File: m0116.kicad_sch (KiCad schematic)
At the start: 259 parts, among them J2 Conn_01x04_MountingPin, J3 Conn_01x04_MountingPin, Q1 Q_PMOS_GSD AO3401A, Q2 Q_NMOS_GSD 2N7002, Q3 Q_NMOS_GSD 2N7002, Q4 2N3904, SW1 SW_Push, U1 XC6206P332MR, U2 74AHCT1G125, U3 STM32F411RETx, U4 24LC64, U5 USBLC6-2SC6, Y1 8MHz

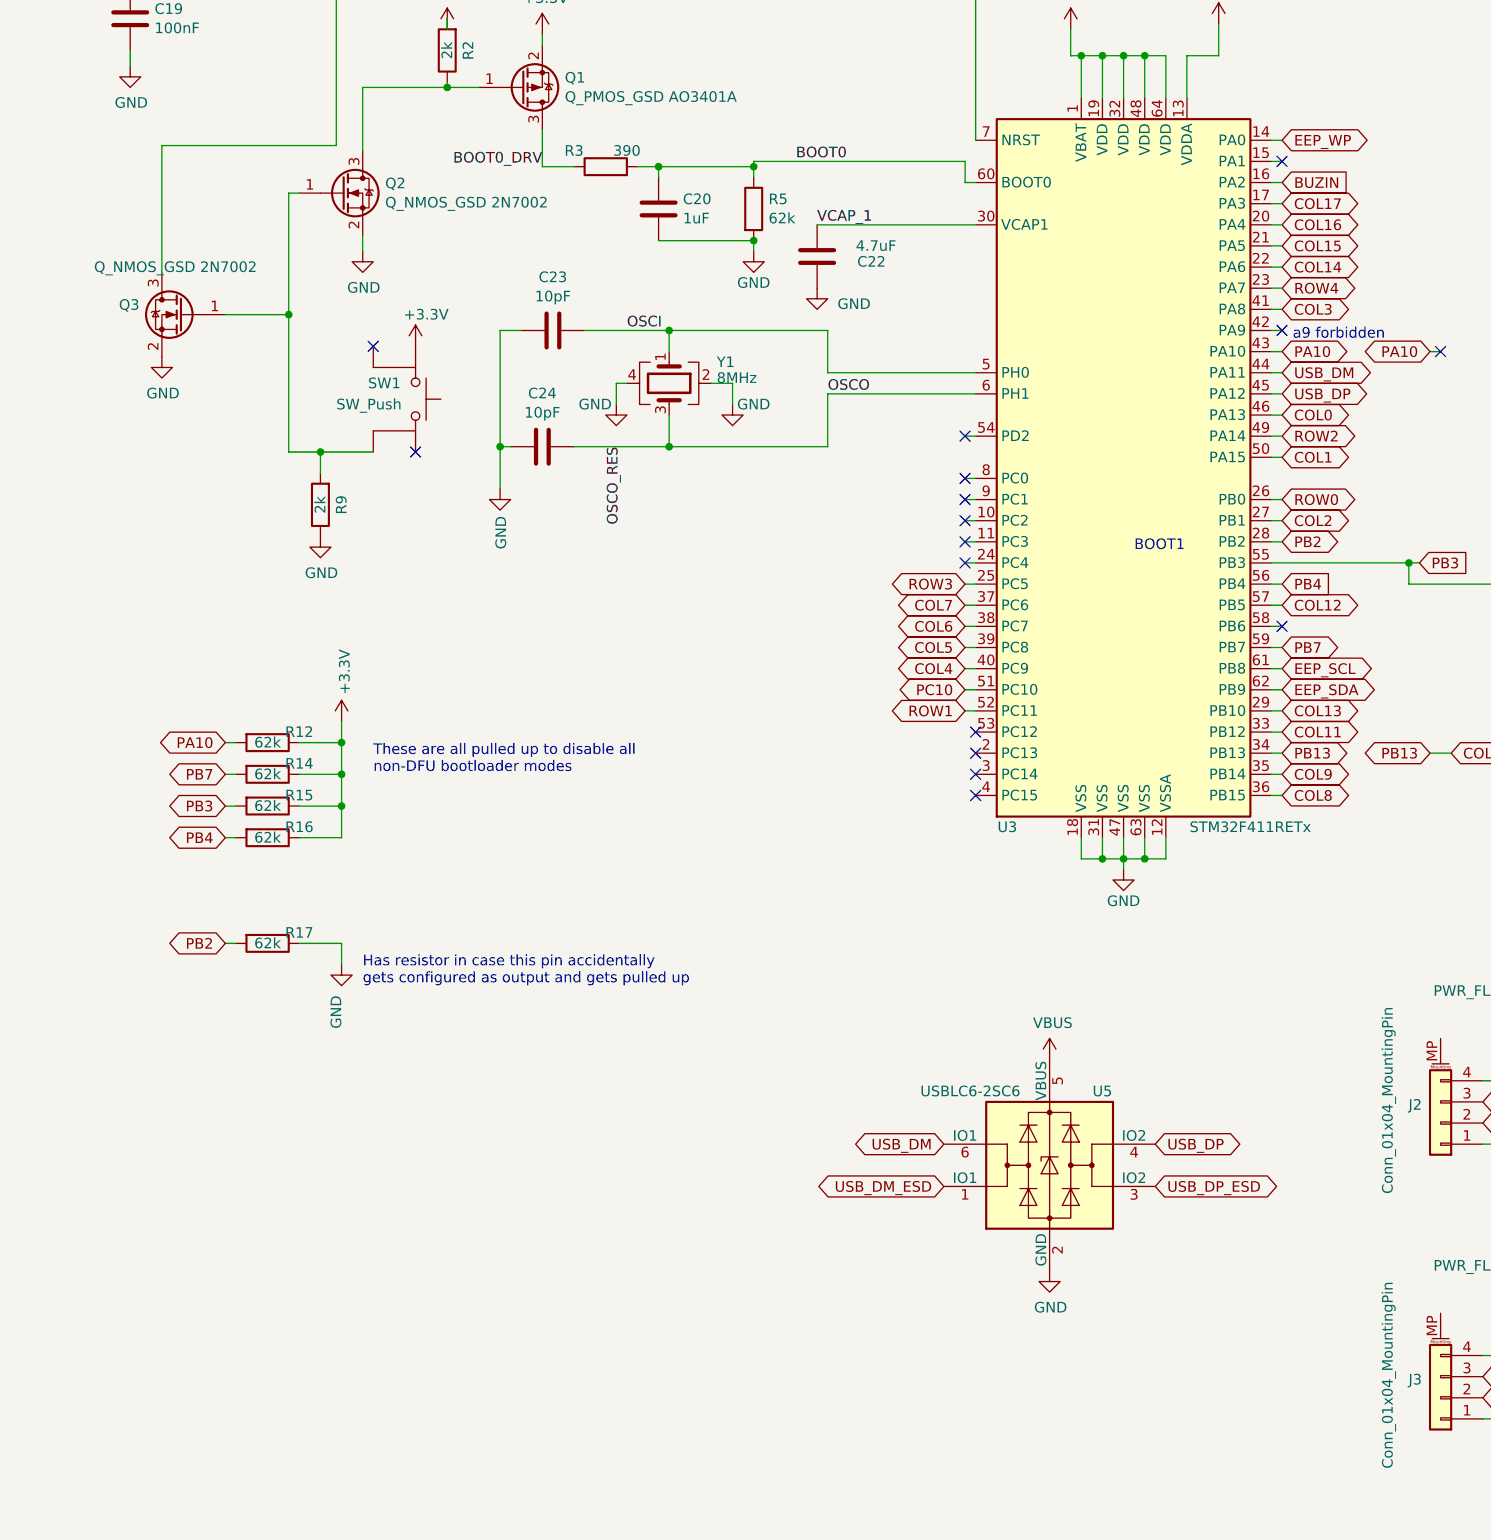
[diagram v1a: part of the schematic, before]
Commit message: updates
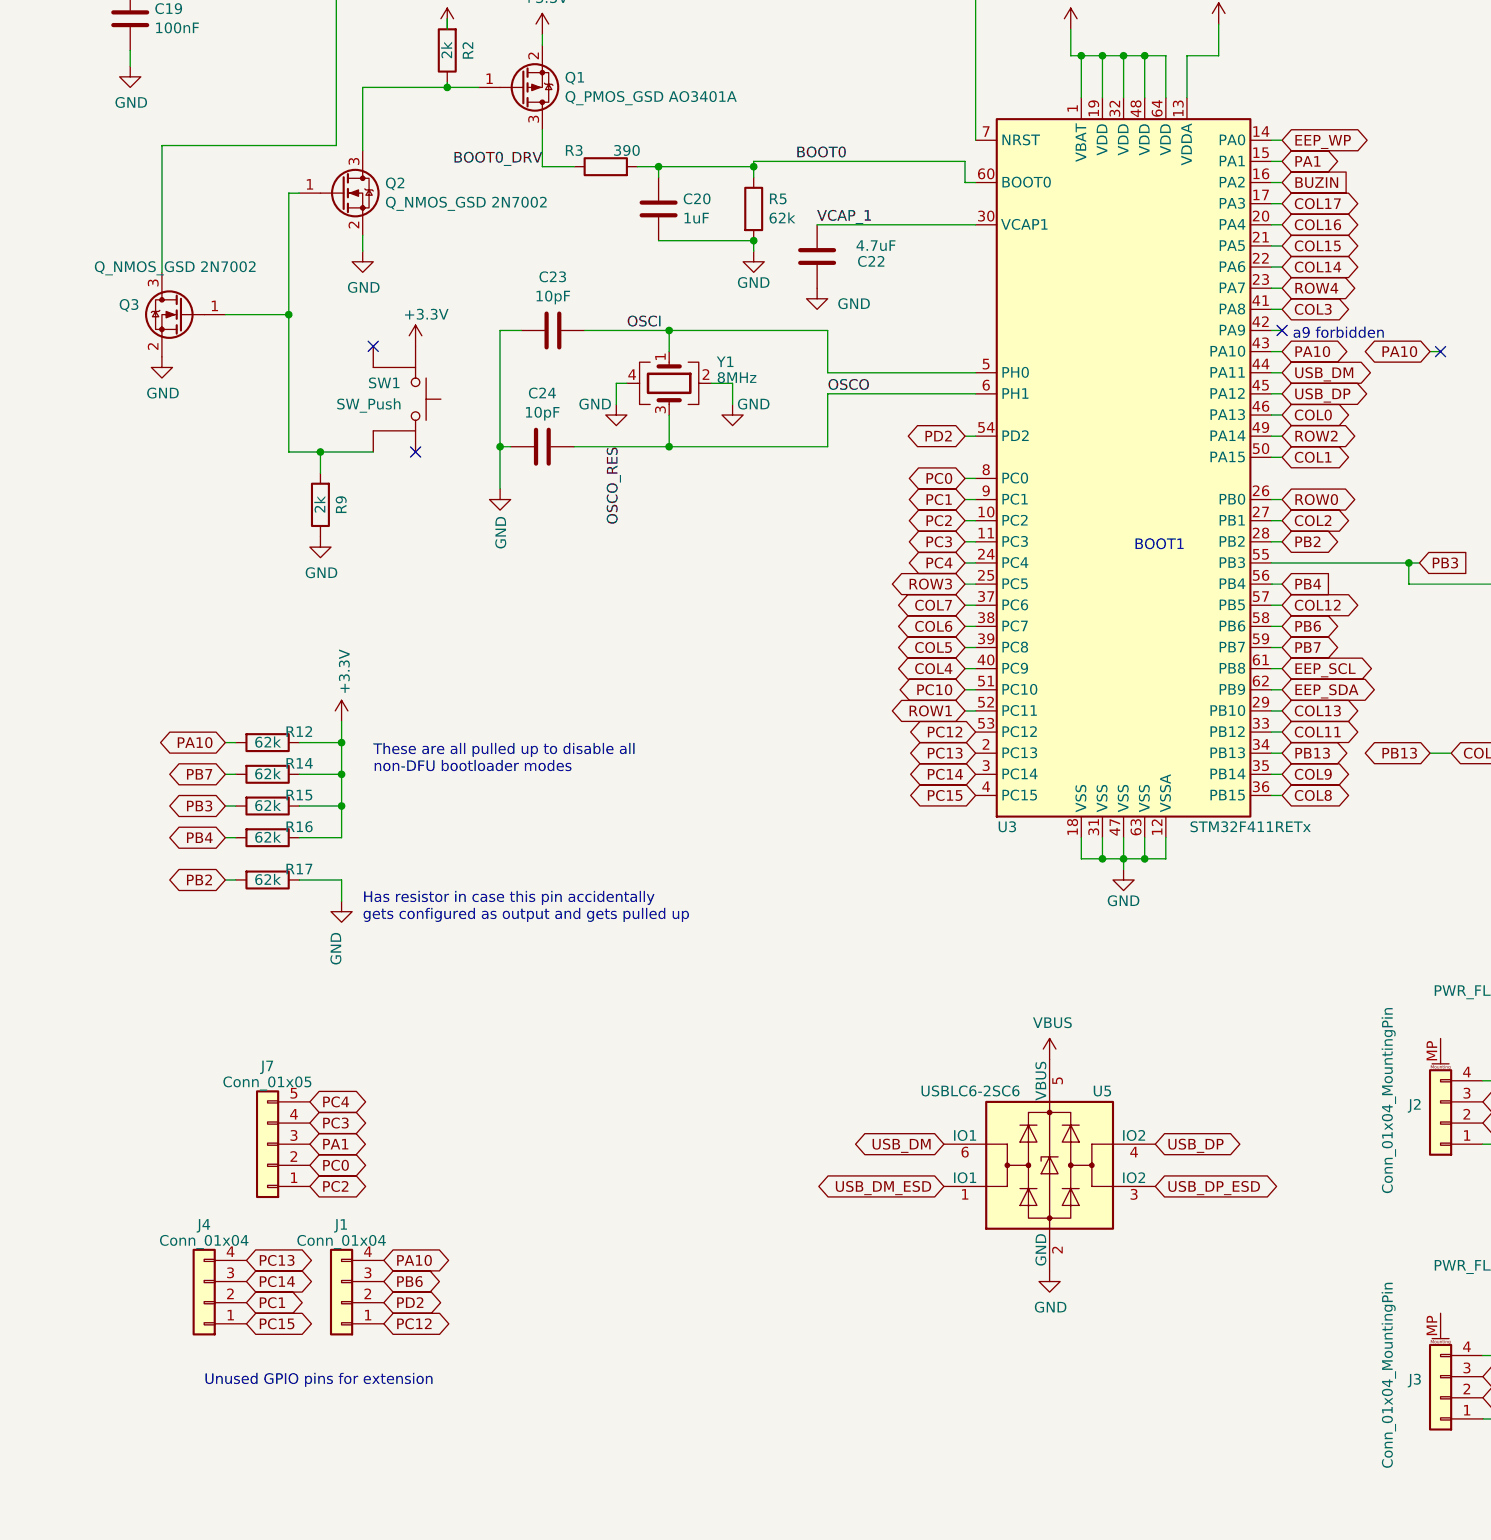
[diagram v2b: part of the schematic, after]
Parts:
- added J1, J4: Conn_01x04, Connector_PinHeader_1.27mm:PinHeader_1x04_P1.27mm_Vertical, symbol Connector_Generic:Conn_01x04
- added J7: Conn_01x05, Connector_PinHeader_1.27mm:PinHeader_1x05_P1.27mm_Vertical, symbol Connector_Generic:Conn_01x05
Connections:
- net PA10: now also J1.4 (Pin_4)
- net PC2: now reaches U3.10 (PC2)
- net PC2: now also J7.1 (Pin_1)
- net PC3: now reaches U3.11 (PC3)
- net PC3: now also J7.4 (Pin_4)
- net PA1: now reaches U3.15 (PA1)
- net PA1: now also J7.3 (Pin_3)
- net PC13: now reaches U3.2 (PC13)
- net PC13: now also J4.4 (Pin_4)
- net PC4: now reaches U3.24 (PC4)
- net PC4: now also J7.5 (Pin_5)
- net PC14: now reaches U3.3 (PC14)
- net PC14: now also J4.3 (Pin_3)
- net PC15: now reaches U3.4 (PC15)
- net PC15: now also J4.1 (Pin_1)
- net PC12: now reaches U3.53 (PC12)
- net PC12: now also J1.1 (Pin_1)
- net PD2: now reaches U3.54 (PD2)
- net PD2: now also J1.2 (Pin_2)
- net PB6: now reaches U3.58 (PB6)
- net PB6: now also J1.3 (Pin_3)
- net PC0: now reaches U3.8 (PC0)
- net PC0: now also J7.2 (Pin_2)
- net PC1: now reaches U3.9 (PC1)
- net PC1: now also J4.2 (Pin_2)
- no-connect marks 16 -> 4
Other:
- note added: "Unused GPIO pins for extension"
- moved on the sheet: R17

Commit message: updates
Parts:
- U5: footprint Package_TO_SOT_SMD:SOT-666 -> Package_TO_SOT_SMD:SOT-23-6; LCSC C15999 -> C7519
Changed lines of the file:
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@@
       (effects (font (size 1.27 1.27)))
     )
-    (property "Footprint" "Package_TO_SOT_SMD:SOT-666" (at 115.57 194.31 0)
+    (property "Footprint" "Package_TO_SOT_SMD:SOT-23-6" (at 115.57 194.31 0)
       (effects (font (size 1.27 1.27)) hide)
     )
@@
       (effects (font (size 1.27 1.27)) hide)
     )
-    (property "LCSC" "C15999" (at 134.62 204.47 0)
+    (property "LCSC" "C7519" (at 134.62 204.47 0)
       (effects (font (size 1.27 1.27)) hide)
     )
